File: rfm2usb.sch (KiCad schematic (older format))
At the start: 23 parts, among them J1 USB_B_Micro, J2 DBG, J4 SMA, J5 UART, U1 AP2210N-3.3TRG1, U2 STM32F042K6Tx, U3 RFM69HCW, Y1 8MHz

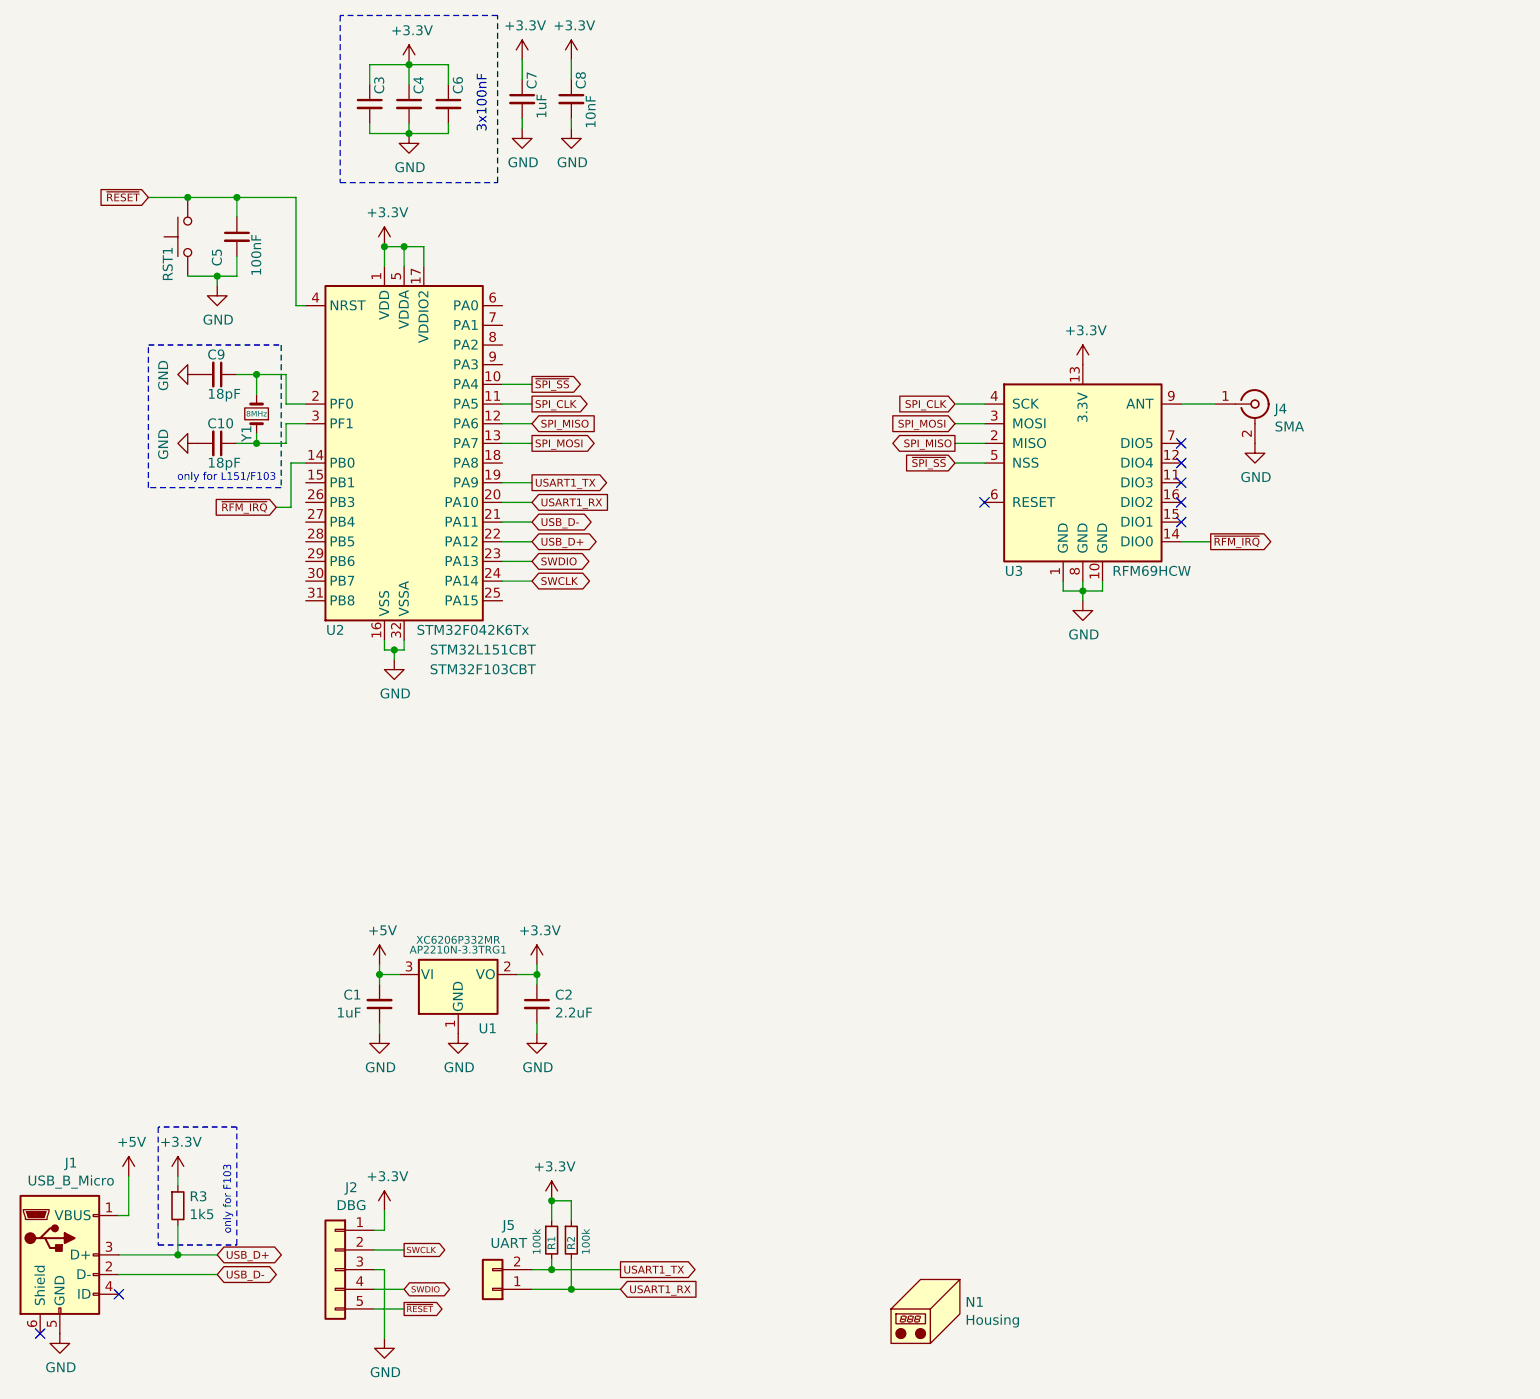
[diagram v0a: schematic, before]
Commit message: cleanup
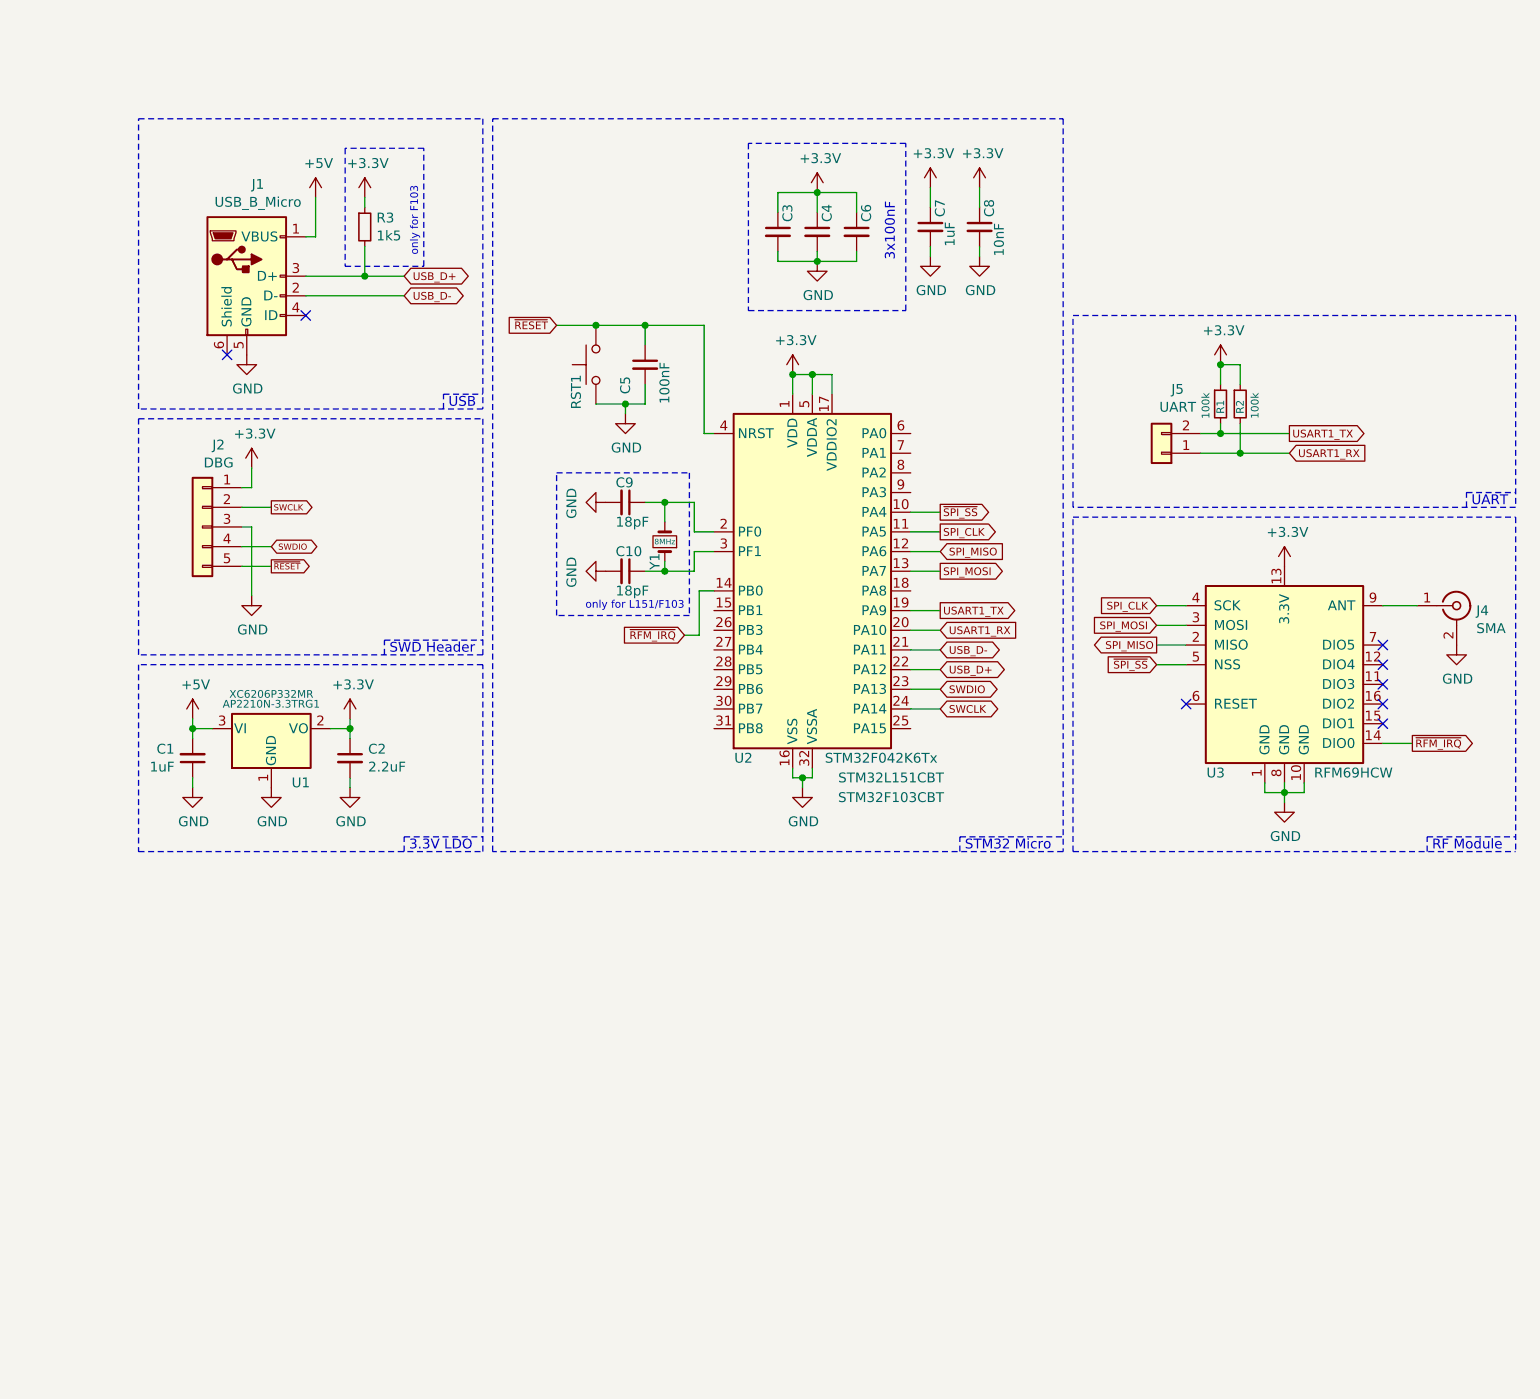
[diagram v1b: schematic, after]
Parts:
- removed N1: Housing, Symbol:KiCad-Logo2_5mm_Copper, symbol Mechanical:Housing
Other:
- note added: "3.3V LDO"
- note added: "RF Module"
- note added: "STM32 Micro"
- note added: "SWD Header"
- note added: "UART"
- note added: "USB"
- moved on the sheet: C1, C10, C2, C3, C4, C5, C6, C7, C8, C9, J1, J2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
